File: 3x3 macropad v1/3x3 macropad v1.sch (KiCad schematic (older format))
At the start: 34 parts, among them SW1 SW_Push, U1 ATmega32U4-AU, Y1 16MHz

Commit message: Added images
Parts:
- removed MX1, MX2, MX3, MX4, MX5, MX6, MX7, MX8, MX9: MX-NoLED, MX_Alps_Hybrid_Laptop:MX-1U, symbol first-keyboard-rescue:MX-NoLED-MX_Alps_Hybrid_Laptop
- removed USB1: Molex-0548190589, random-keyboard-parts:Molex-0548190589, symbol first-keyboard-rescue:Molex-0548190589-random-keyboard-parts_Laptop
- added MX1, MX2, MX3, MX4, MX5, MX6, MX7, MX8, MX9: MX-NoLED, symbol MX_Alps_Hybrid:MX-NoLED
- added USB1: Molex-0548190589, symbol random-keyboard-parts:Molex-0548190589
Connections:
- wire segments 80 -> 79
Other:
- moved on the sheet: C1, C2, C3, C4, C5, C6, C7, D1, D2, D3, D4, D5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

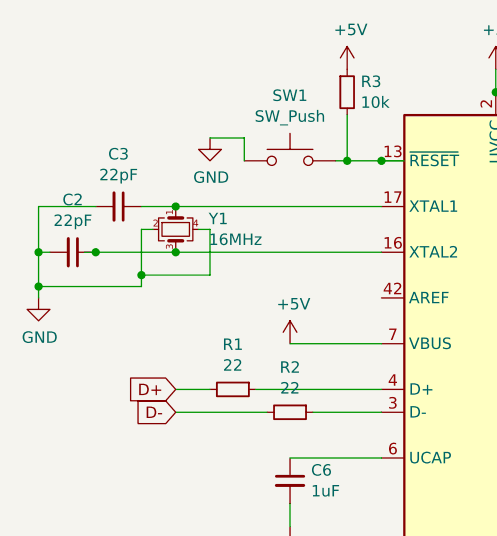
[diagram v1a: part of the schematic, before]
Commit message: numpad/5x5 macropad project
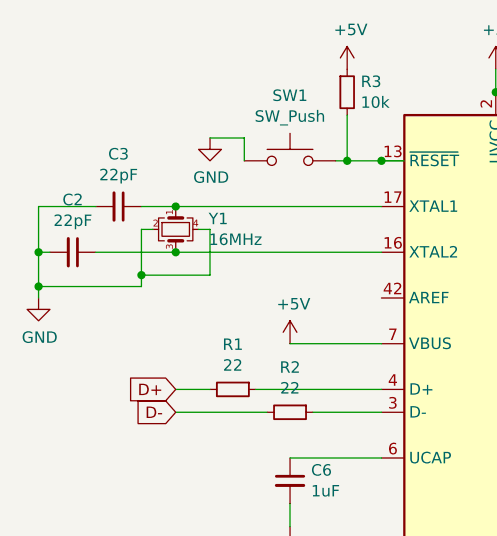
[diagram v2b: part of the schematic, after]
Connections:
- wire segments 79 -> 78
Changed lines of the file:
@@
 EESchema Schematic File Version 4
+LIBS:3x3 macropad v1-cache
 EELAYER 29 0
 EELAYER END
@@
 $EndComp
 Connection ~ 1850 2200
-Wire Wire Line
-	1450 2400 1500 2400
 Connection ~ 1850 2400
 Wire Wire Line
@@
 Wire Wire Line
 	1700 2200 1850 2200
-Connection ~ 1500 2400
 Wire Wire Line
 	1250 2200 1500 2200
